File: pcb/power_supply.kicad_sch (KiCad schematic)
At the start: 34 parts

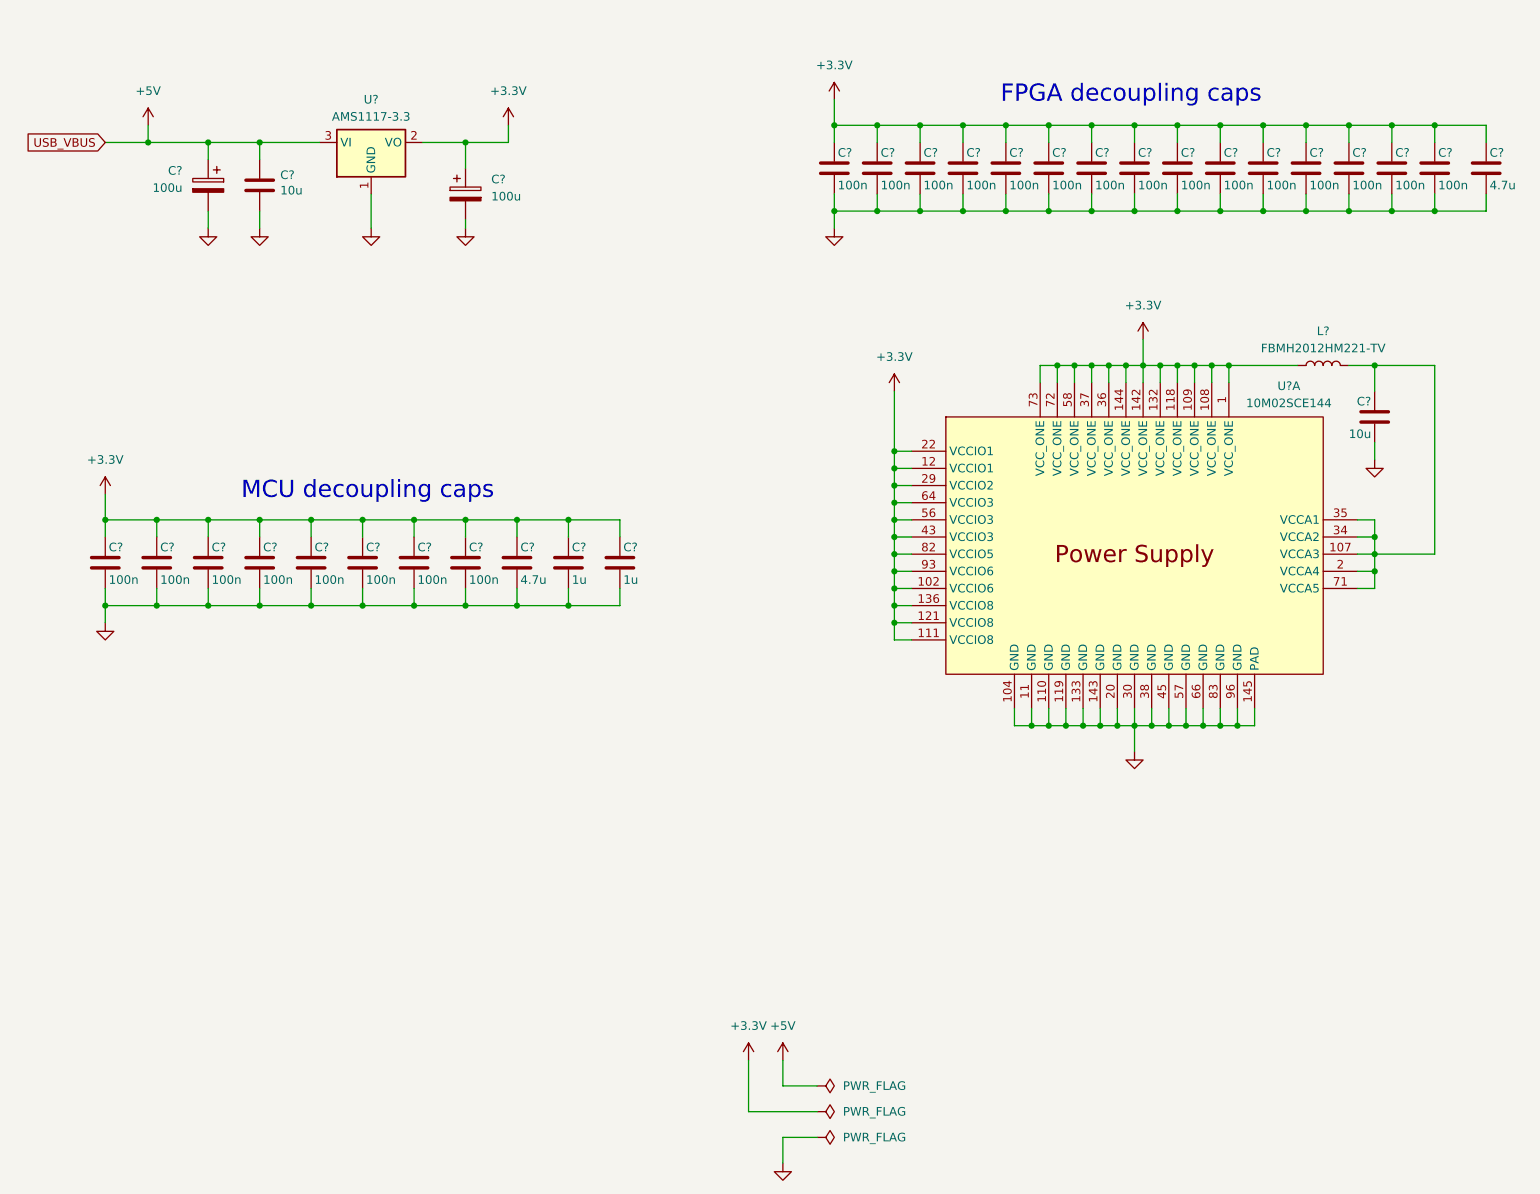
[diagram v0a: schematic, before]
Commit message: Further schematic capture
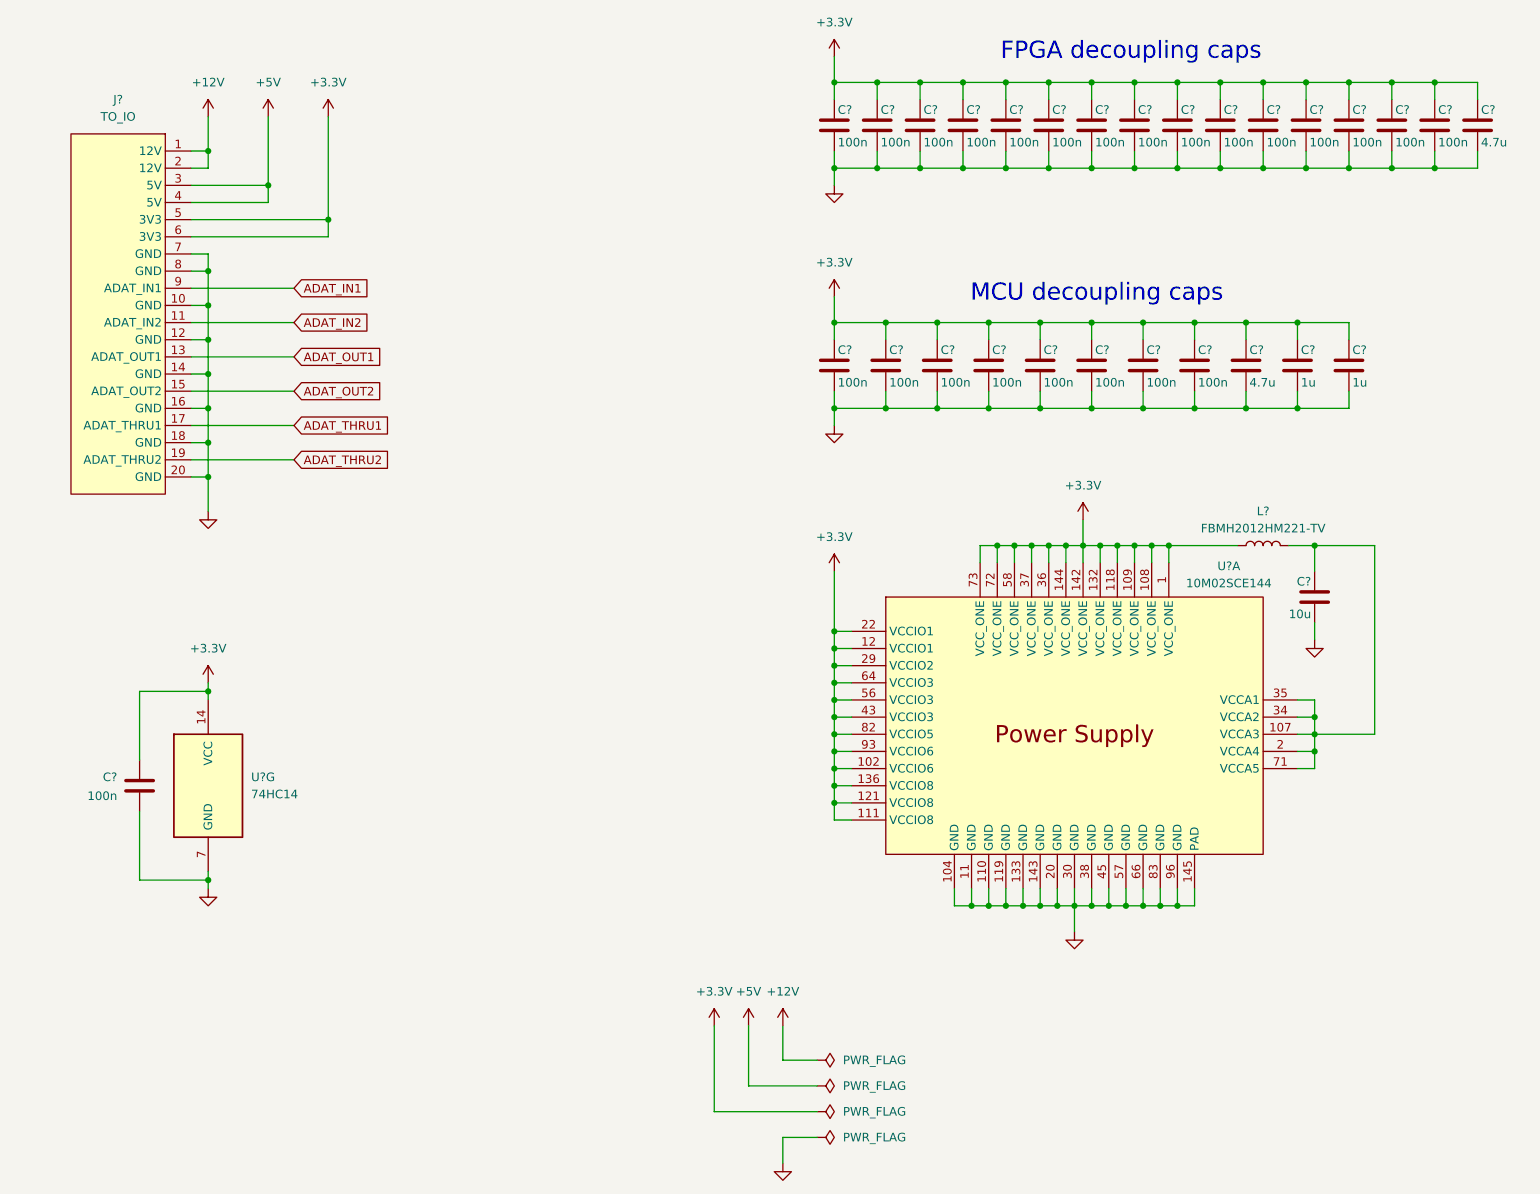
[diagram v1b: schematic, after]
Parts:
- removed C? (x2): 100u, symbol Device:C_Polarized
- removed C?: 10u, symbol Device:C
- removed U?: AMS1117-3.3, Package_TO_SOT_SMD:SOT-223-3_TabPin2, symbol Regulator_Linear:AMS1117-3.3
- added C?: 100n, symbol Device:C
- added J?: TO_IO, symbol adatv2:Connector_IO
- added U?: 74HC14, symbol 74xx:74HC14
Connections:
- net +3.3V: now also C?.1, J?.5 (3V3), J?.6 (3V3), U?.14 (VCC)
- net +5V: now also J?.3 (5V), J?.4 (5V)
- net GND: now also C?.2, U?.7 (GND)
- new net +12V: J?.1 (12V), J?.2 (12V)
- new net ADAT_IN1: J?.9 (ADAT_IN1)
- new net ADAT_IN2: J?.11 (ADAT_IN2)
- new net ADAT_OUT1: J?.13 (ADAT_OUT1)
- new net ADAT_OUT2: J?.15 (ADAT_OUT2)
- new net ADAT_THRU1: J?.17 (ADAT_THRU1)
- new net ADAT_THRU2: J?.19 (ADAT_THRU2)
- new net GND_IO: J?.10 (GND), J?.12 (GND), J?.14 (GND), J?.16 (GND), J?.18 (GND), J?.20 (GND), J?.7 (GND), J?.8 (GND)
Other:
- moved on the sheet: C?, L?, U?A
